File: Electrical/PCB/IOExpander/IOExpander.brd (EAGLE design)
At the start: 38 parts, among them U1 MCP23017T-E/SS

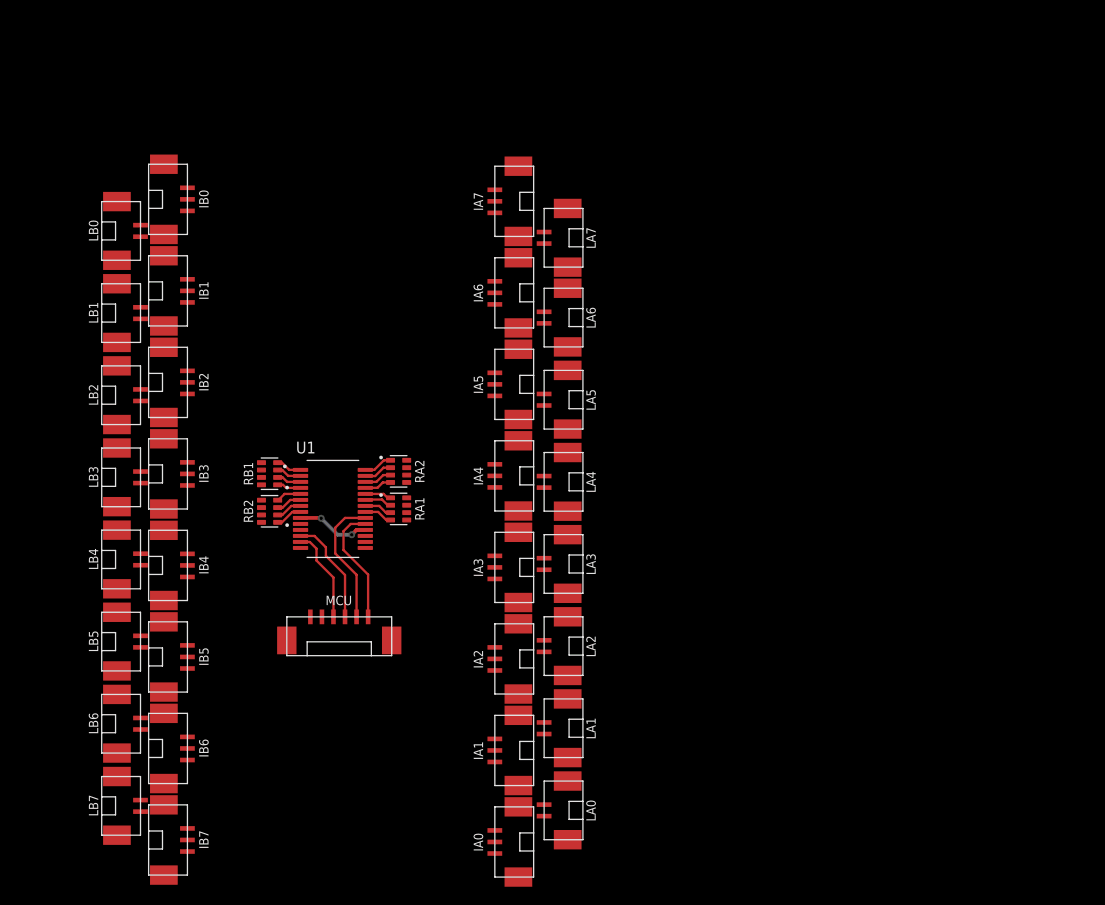
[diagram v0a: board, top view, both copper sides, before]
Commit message: PCB Batch #1
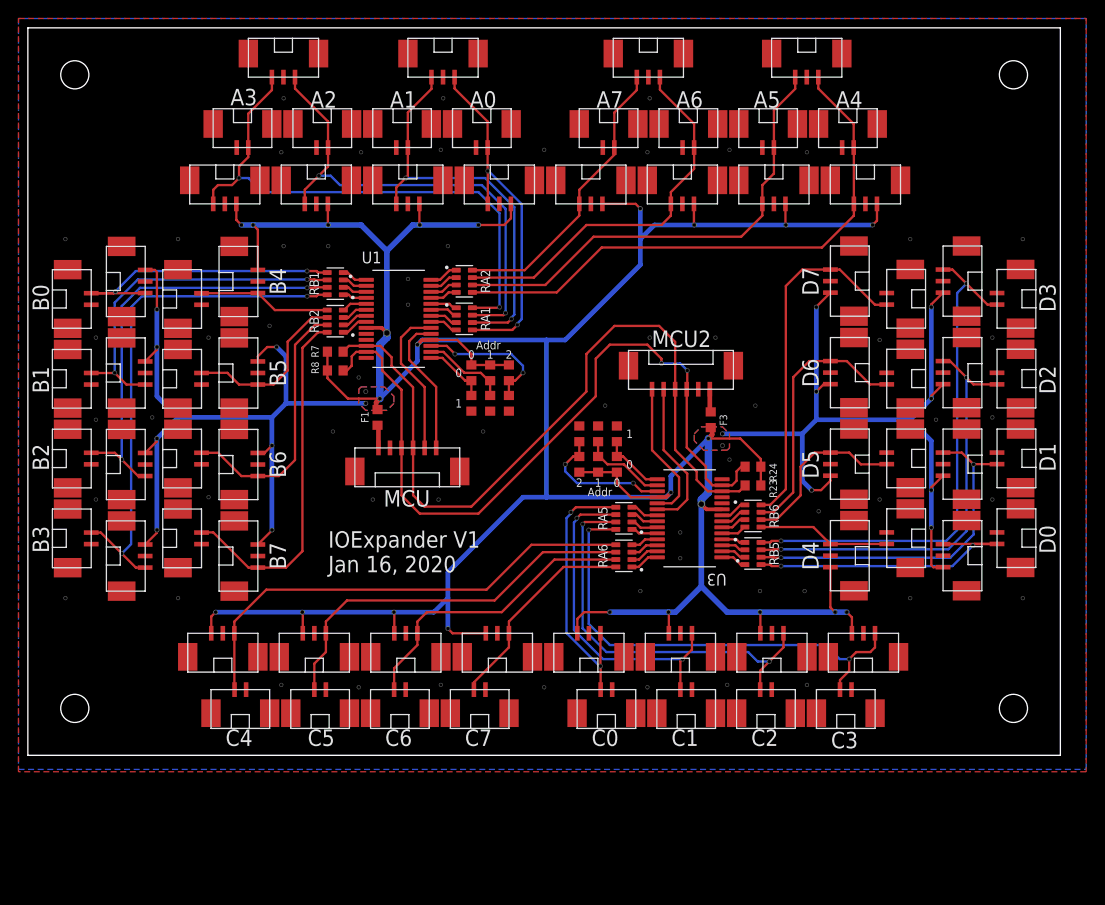
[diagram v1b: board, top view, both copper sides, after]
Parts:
- added A0A1, A2A3, A4A5, A6A7, IA16, IA17, IA18, IA19, IA20, IA21, IA22, IA23, IB16, IB17, IB18, IB19, IB20, IB21, IB22, IB23: JST_1.25_3P, Scott-Connectors:JST1.25_3P
- added F1, F3: (no value), Scott-Electrical:0603
- added H1, H2, H3, H4: HOLE-M3, Scott-Mechanical:M3
- added LA16, LA17, LA18, LA19, LA20, LA21, LA22, LA23, LB16, LB17, LB18, LB19, LB20, LB21, LB22, LB23: JST_1.25_2P, Scott-Connectors:JST1.25_2P
- added MCU2: JST_1.25_6P, Scott-Connectors:JST1.25_6P
- added R1, R17, R19, R21, R23, R24, R3, R5, R7, R8: DNP, Scott-Electrical:0603
- added R18, R2, R20, R22, R4, R6: 10K, Scott-Electrical:0603
- added RA5, RA6, RB5, RB6: (no value), Scott-Electrical:RESCAF80P320X160X60-8N
- added U3: MCP23017T-E/SS, Scott-ICs:SOP65P780X200-28N
- moved LA0 71.5 mm to (48.5, 65.8), turned to 0 degrees
- moved IA0 67.8 mm to (49.8, 59.7), turned to 0 degrees
- moved LA1 64.3 mm to (39.9, 65.8), turned to 0 degrees
- moved IA1 58.9 mm to (39.9, 59.7), turned to 0 degrees
- moved LA2 58.8 mm to (31.2, 65.8), turned to 0 degrees
- moved LA3 55.5 mm to (22.6, 65.8), turned to 0 degrees
- moved IA2 52.2 mm to (30.0, 59.7), turned to 0 degrees
- moved IA3 48.8 mm to (20.1, 59.7), turned to 0 degrees
- moved IA4 48.0 mm to (89.4, 59.7), turned to 0 degrees
- moved LA4 48.0 mm to (88.1, 65.8), turned to 0 degrees
- moved LA5 35.6 mm to (79.5, 65.8), turned to 0 degrees
- moved IA5 34.2 mm to (79.5, 59.7), turned to 0 degrees
- moved IB7 31.7 mm to (24.9, 20.3)
- moved IB4 31.7 mm to (24.9, 50.0)
- moved IB5 31.7 mm to (24.9, 40.1)
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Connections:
- new net ADDR0: R1.1, R2.2, U1.15
- new net ADDR0_2: R17.1, R18.2, U3.15
- new net ADDR1: R3.1, R4.2, U1.16
- new net ADDR1_2: R19.1, R20.2, U3.16
- new net ADDR2: R5.1, R6.2, U1.17
- new net ADDR2_2: R21.1, R22.2, U3.17
- new net C0: IA23.1, LA23.2, RA5.5
- new net C1: IA16.1, LA16.2, RA5.6
- new net C2: IA17.1, LA17.2, RA5.7
- new net C3: IA18.1, LA18.2, RA5.8
- new net C4: IA19.1, LA19.2, RA6.5
- new net C5: IA20.1, LA20.2, RA6.6
- new net C6: IA21.1, LA21.2, RA6.7
- new net C7: IA22.1, LA22.2, RA6.8
- new net D0: IB23.1, LB23.2, RB5.5
- new net D1: IB16.1, LB16.2, RB5.6
- new net D2: IB17.1, LB17.2, RB5.7
- new net D3: IB18.1, LB18.2, RB5.8
- new net D4: IB19.1, LB19.2, RB6.5
- new net D5: IB20.1, LB20.2, RB6.6
- new net D6: IB21.1, LB21.2, RB6.7
- new net D7: IB22.1, LB22.2, RB6.8
- new net INTC: MCU2.2, U3.20
- new net INTD: MCU2.1, U3.19
- new net N$35: RB5.1, U3.4
- new net N$36: RB5.2, U3.3
- new net N$37: RB5.3, U3.2
- new net N$38: RB5.4, U3.1
- new net N$39: RB6.1, U3.8
- new net N$40: RB6.2, U3.7
- new net N$41: RB6.3, U3.6
- new net N$42: RB6.4, U3.5
- new net N$43: RA5.1, U3.24
- new net N$46: RA5.4, U3.21
- new net N$47: RA6.1, U3.28
- new net N$48: RA6.2, U3.27
- new net N$49: RA6.3, U3.26
- new net N$50: RA6.4, U3.25
- new net N$51: F3.2, MCU2.6
- new net N$9: F1.2, MCU.6
- net 3.3V: now also F1.1, F3.1, IA16.3, IA17.3, IA18.3, IA19.3, IA20.3, IA21.3, IA22.3, IA23.3, IB0.3, IB1.3, IB16.3, IB17.3, IB18.3, IB19.3, IB2.3, IB20.3, IB21.3, IB22.3, IB23.3, IB3.3, IB4.3, IB5.3, IB6.3, IB7.3, R1.2, R17.2, R19.2, R21.2, R23.1, R24.1, R3.2, R5.2, R7.1, R8.1, U3.18, U3.9; no longer MCU.6
- net A0: now also A0A1.3
- net A1: now also A0A1.1
- net A2: now also A2A3.3
- net A3: now also A2A3.1
- net A4: now also A4A5.3
- net A5: now also A4A5.1
- net A6: now also A6A7.3
- net A7: now also A6A7.1
- net GND: now also A0A1.2, A2A3.2, A4A5.2, A6A7.2, IA16.2, IA17.2, IA18.2, IA19.2, IA20.2, IA21.2, IA22.2, IA23.2, IB0.2, IB1.2, IB16.2, IB17.2, IB18.2, IB19.2, IB2.2, IB20.2, IB21.2, IB22.2, IB23.2, IB3.2, IB4.2, IB5.2, IB6.2, IB7.2, LA16.1, LA17.1, LA18.1, LA19.1, LA20.1, LA21.1, LA22.1, LA23.1, LB16.1, LB17.1, LB18.1, LB19.1, LB20.1, LB21.1, LB22.1, LB23.1, MCU2.5, R18.1, R2.1, R20.1, R22.1, R4.1, R6.1, U3.10; no longer U1.15, U1.16, U1.17
- net N$44: now also RA5.2, U3.23; no longer IB0.3, IB1.3, IB2.3, IB3.3, IB4.3, IB5.3, IB6.3, IB7.3
- net N$45: now also RA5.3, U3.22; no longer IB0.2, IB1.2, IB2.2, IB3.2, IB4.2, IB5.2, IB6.2, IB7.2
- net SCL: now also MCU2.3, R23.2, R7.2, U3.12
- net SDA: now also MCU2.4, R24.2, R8.2, U3.13
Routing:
- net 3.3V: track 7.98 -> 516.6 mm, vias 2 -> 42
- net SDA: track 10.2 -> 83.3 mm, vias 0 -> 2
- net SCL: track 11.6 -> 83.9 mm
- net A4: track 0.00 -> 61.3 mm
- net A3: track 0.00 -> 60.1 mm, vias 0 -> 2
- net D3: track 0.00 -> 56.3 mm, vias 0 -> 2
- net B3: track 0.00 -> 56.3 mm, vias 0 -> 2
- net A2: track 0.00 -> 52.9 mm, vias 0 -> 2
- net C4: track 0.00 -> 52.1 mm
- net C3: track 0.00 -> 51.5 mm, vias 0 -> 2
- net A5: track 0.00 -> 51.0 mm
- net B2: track 0.00 -> 46.6 mm, vias 0 -> 2
- net D2: track 0.00 -> 46.6 mm, vias 0 -> 2
- net A1: track 0.00 -> 45.0 mm, vias 0 -> 2
- net C2: track 0.00 -> 43.8 mm, vias 0 -> 2
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- added copper zone on layer 1, net 3.3V
- added copper zone on layer 16, net 3.3V
- added copper zone on layer 1, net GND
- added copper zone on layer 16, net GND
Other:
- board outline added: 111.8 x 78.7 mm
- board text added: "0"
- board text added: "1"
- board text added: "2"
- board text added: "A0"
- board text added: "A1"
- board text added: "A2"
- board text added: "A3"
- board text added: "A4"
- board text added: "A5"
- board text added: "A6"
- board text added: "A7"
- board text added: "Addr"
- board text added: "B0"
- board text added: "B1"
- board text added: "B2"
- board text added: "B3"
- board text added: "B4"
- board text added: "B5"
- board text added: "B6"
- board text added: "B7"
- board text added: "C0"
- board text added: "C1"
- board text added: "C2"
- board text added: "C3"
- board text added: "C4"
- board text added: "C5"
- board text added: "C6"
- board text added: "C7"
- board text added: "D0"
- board text added: "D1"
- board text added: "D2"
- board text added: "D3"
- board text added: "D4"
- board text added: "D5"
- board text added: "D6"
- board text added: "D7"
- board text added: "IOExpander V1 Jan 16, 2020"
